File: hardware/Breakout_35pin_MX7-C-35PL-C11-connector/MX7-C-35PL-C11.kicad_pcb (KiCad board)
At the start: 2 copper layers, 47 x 35.6 mm, 13 parts, among them P1 CONN_1, P10 CONN_01X02, P11 CONN_01X08, P12 CONN_01X02, P13 CONN_01X02, P2 CONN_1, P3 CONN_01X02, P4 CONN_01X02, P5 CONN_01X07, P6 CONN_01X02, P7 CONN_01X04, P8 MX7-C-35PL-C11, P9 CONN_01X04

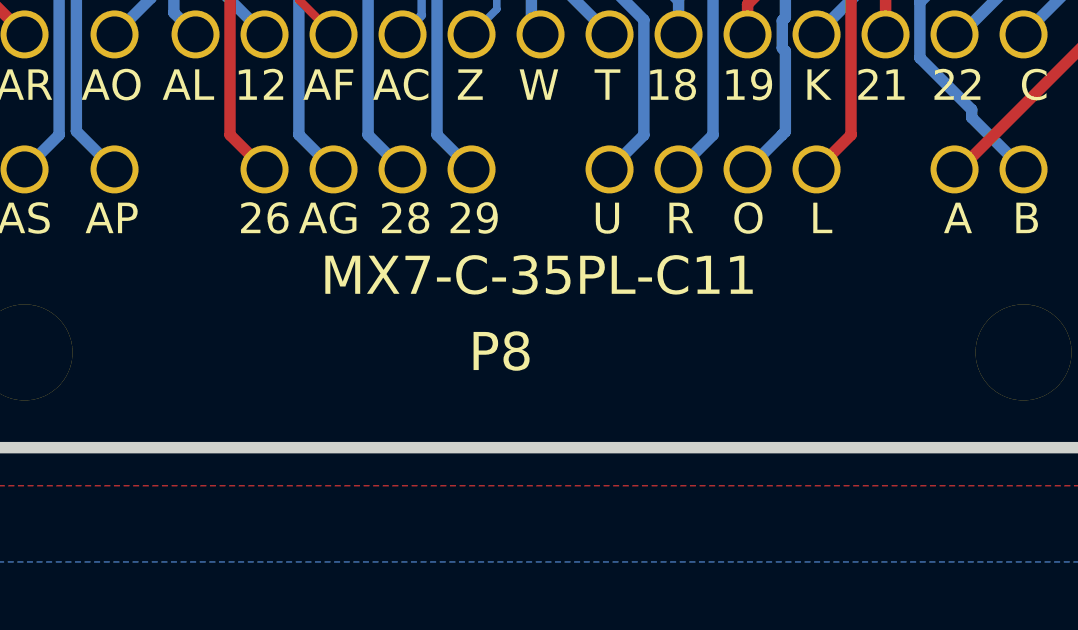
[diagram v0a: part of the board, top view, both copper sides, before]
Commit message: update pcb files
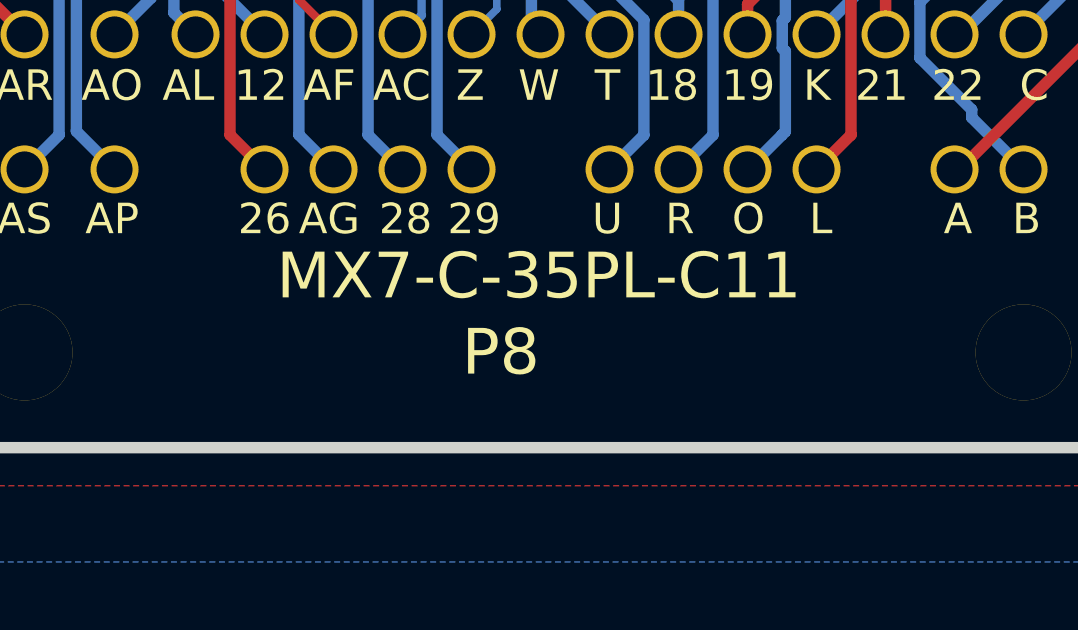
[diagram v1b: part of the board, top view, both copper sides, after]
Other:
- net class Default removed
